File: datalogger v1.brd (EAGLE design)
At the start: 82.5 x 67 mm, 15 parts, among them M1 ARDUINO-NANO-3.0#ISP

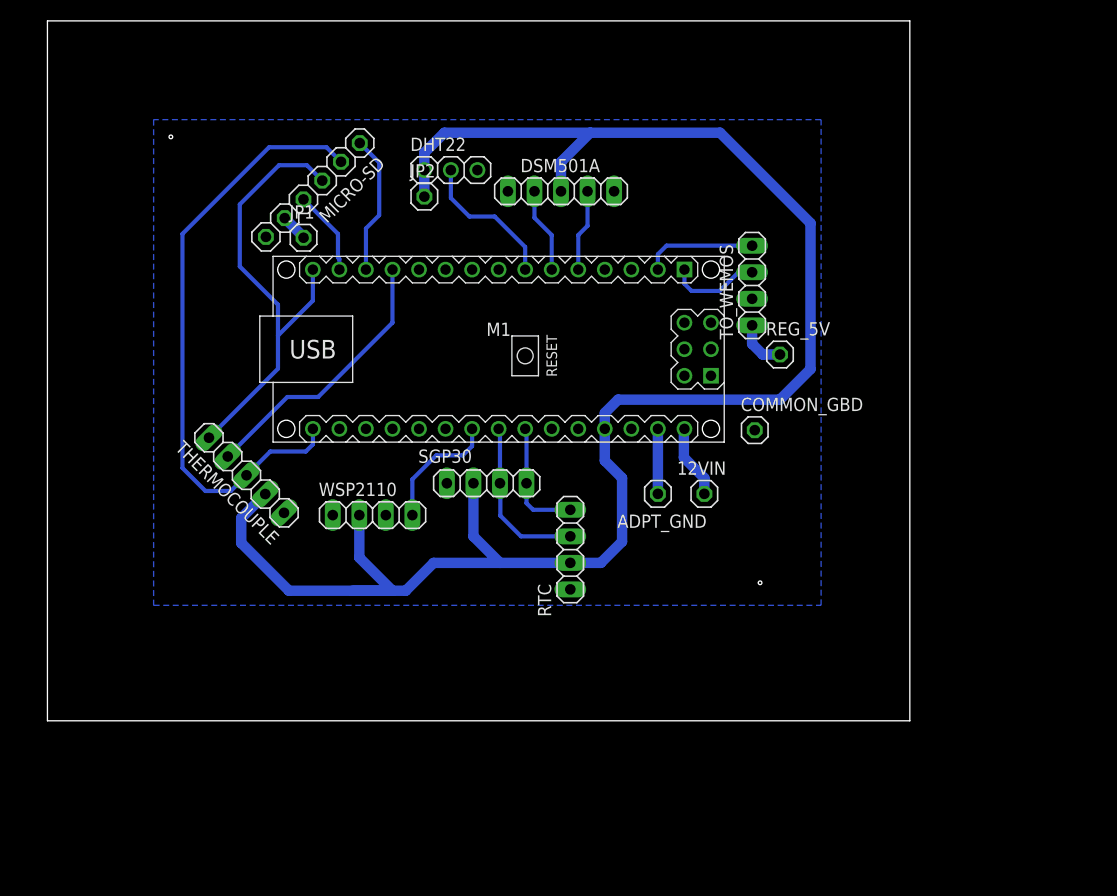
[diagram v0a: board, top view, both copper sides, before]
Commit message: final
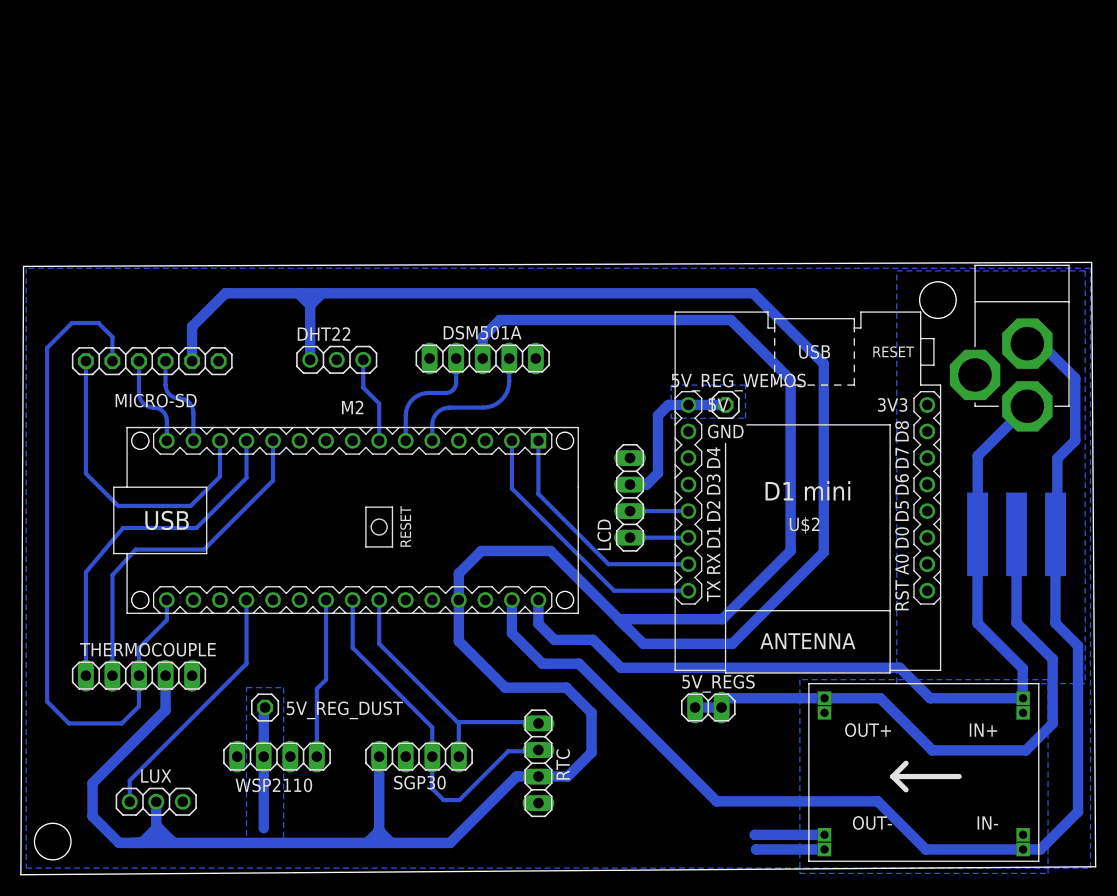
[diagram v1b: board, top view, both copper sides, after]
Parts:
- removed 12VIN, ADPT_GND, COMMON_GBD, JP1, JP2, REG_5V: (no value), pinhead:1X01
- removed M1: ARDUINO-NANO-3.0#ISP, diy-modules:ARDUINO-NANO-3.0#ISP
- removed TO_WEMOS: (no value), pinhead:1X04
- added 5V_REGS: (no value), pinhead:1X02
- added 5V_REG_DUST, 5V_REG_WEMOS: (no value), pinhead:1X01
- added LCD: (no value), pinhead:1X04
- added LUX: (no value), adafruit:1X03
- added M2: ARDUINO-NANO-3.0, diy-modules:ARDUINO-NANO-3.0
- added U$1: MP1584, MP1584-dc-brick:DC-BRICK
- added U$2: WEMOS-D1-MINI, diy-modules:WEMOS-D1-MINI
- added U$3: EDGE_CONNECTOR, P_Dusk:EDGE_CONNECTOR
- added X1: (no value), power-jack:DC-21MM
- moved SGP30 27.0 mm to (43.2, 11.8)
- moved WSP2110 24.9 mm to (29.6, 11.8)
- moved MICRO-SD 22.5 mm to (17.7, 49.7), turned to 180 degrees
- moved THERMOCOUPLE 21.8 mm to (16.4, 19.6), turned to 180 degrees
- moved DHT22 21.2 mm to (35.3, 49.8)
- moved RTC 20.7 mm to (54.6, 11.2)
- moved DSM501A 17.7 mm to (49.3, 49.9)
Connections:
- removed net 12V_ADP: 12VIN.1, M1.J2.1
- new net 1: X1.1
- new net 12V: M2.J2.1, U$1.IN1+, U$1.IN2+, U$3.12V, X1.2
- new net D_THERMO: M2.J1.12, THERMOCOUPLE.5
- new net LUX_A: LUX.1, M2.J2.12
- new net SCL_LCD: LCD.1, U$2.JP2.3
- new net SDA_LCD: LCD.2, U$2.JP2.4
- net 3V3: now also M2.J2.14, U$2.JP1.8; no longer M1.J2.14
- net 5V: now also LUX.2, M2.J2.4, SGP30.1; no longer JP1.1, JP2.1, M1.J2.4, SGP30.2, WSP2110.2
- net 5V_REG: now also 5V_REGS.1, 5V_REGS.2, 5V_REG_DUST.1, 5V_REG_WEMOS.1, LCD.3, U$1.OUT1+, U$1.OUT2+, U$2.JP2.8, U$3.5V, WSP2110.2; no longer REG_5V.1, TO_WEMOS.1
- net CLK: now also M2.J2.15; no longer M1.J2.15
- net CS: now also M2.J1.13; no longer M1.J1.13
- net CS_THERMO: now also M2.J1.11; no longer M1.J1.12
- net DATA-DHT22: now also DHT22.3, M2.J1.7; no longer DHT22.2, M1.J1.7
- net GND: now also DHT22.2, LCD.4, LUX.3, M2.J1.4, SGP30.2, U$1.OUT1-, U$1.OUT2-, U$2.JP2.7; no longer COMMON_GBD.1, DHT22.3, M1.J1.4, SGP30.1, TO_WEMOS.2
- net GND_ADP: now also M2.J2.2, U$1.IN1-, U$1.IN2-, U$3.GND, X1.3; no longer ADPT_GND.1, M1.J2.2
- net MISO: now also M2.J1.14; no longer M1.J1.14
- net MOSI: now also M2.J1.15; no longer M1.J1.15, THERMOCOUPLE.5
- net RX_WEMOS: now also M2.J1.1, U$2.JP2.2; no longer M1.J1.1, TO_WEMOS.3
- net SCL: now also M2.J2.7; no longer M1.J2.7
- net SDA: now also M2.J2.8; no longer M1.J2.8
- net SIG: now also M2.J2.9; no longer M1.J2.9
- net TX_WEMOS: now also M2.J1.2, U$2.JP2.1; no longer M1.J1.2, TO_WEMOS.4
- net VOUT-1: now also M2.J1.5; no longer M1.J1.5
- net VOUT-2: now also M2.J1.6; no longer M1.J1.6
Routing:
- net 5V: track 170.3 -> 323.6 mm
- net GND_ADP: track 6.22 -> 116.1 mm
- net 12V: track 0.00 -> 83.6 mm
- net 5V_REG: track 4.87 -> 84.4 mm
- net MOSI: track 44.3 -> 8.72 mm
- net D_THERMO: track 0.00 -> 32.8 mm
- net LUX_A: track 0.00 -> 23.9 mm
- net SDA: track 15.9 -> 33.9 mm
- net CS: track 13.5 -> 29.5 mm
- net TX_WEMOS: track 10.8 -> 25.5 mm
- net SCL: track 11.6 -> 26.3 mm
- net RX_WEMOS: track 8.86 -> 22.2 mm
- net GND: track 0.00 -> 13.2 mm
- net CLK: track 58.3 -> 65.6 mm
- net 12V_ADP: track 7.06 -> 0.00 mm
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- added copper zone on layer 16, net NONE
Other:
- board size 82.5 x 67 mm -> 102.9 x 58.6 mm
